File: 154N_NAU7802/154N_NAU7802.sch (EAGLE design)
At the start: 27 parts, among them IC1 MCP604SL, IC2 NAU7802SGI, J4 1725698, J5 1725698, U3 NAU7802, U4 LMV324

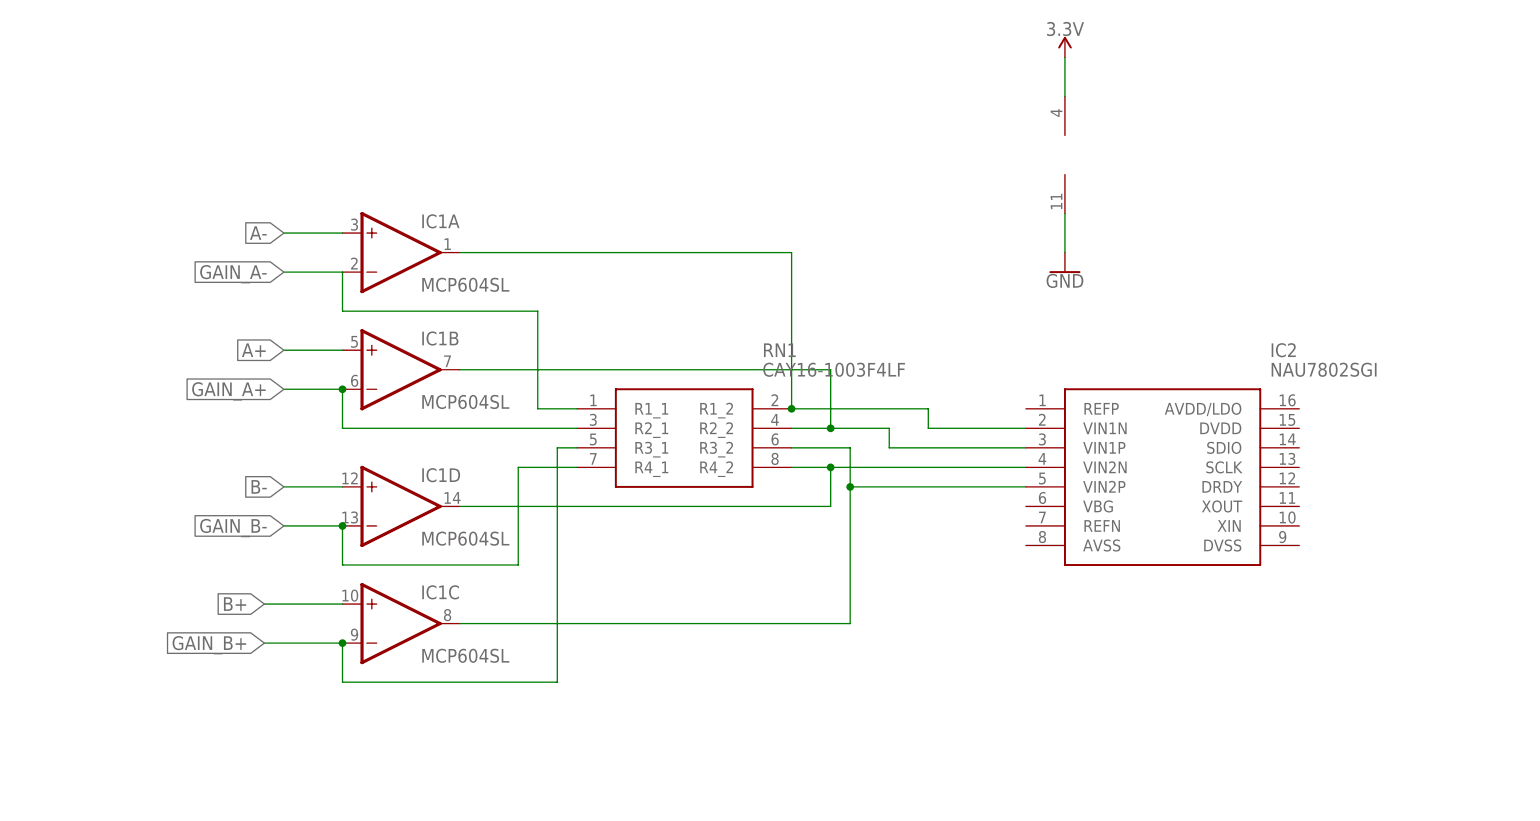
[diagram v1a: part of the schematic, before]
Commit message: Lagopus 3 mm.
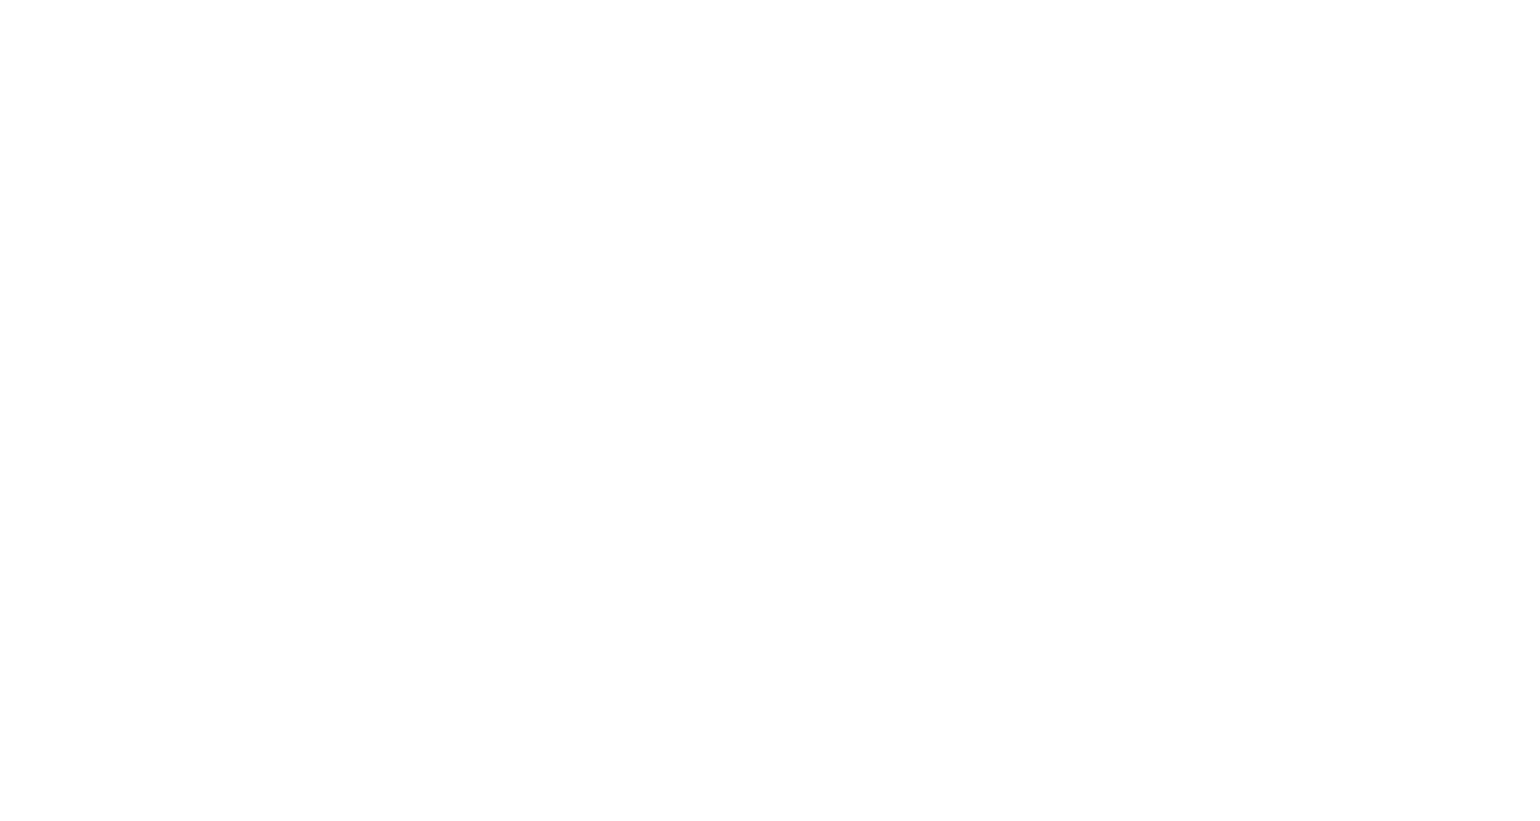
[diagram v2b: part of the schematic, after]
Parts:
- removed IC1: MCP604SL, linear:MCP604SL
- removed IC2: NAU7802SGI, NAU7802SGI:NAU7802SGI
- removed RN1: CAY16-1003F4LF, CAY16-1003F4LF:CAY16-1003F4LF
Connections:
- removed net N$16: IC1C.OUT, IC2.VIN2P, RN1.R3_2
- removed net N$5: IC1A.OUT, IC2.VIN1N, RN1.R1_2
- removed net N$7: IC1B.OUT, IC2.VIN1P, RN1.R2_2
- removed net N$8: IC1D.OUT, IC2.VIN2N, RN1.R4_2
- net 3.3V: no longer IC1P.V+
- net A+: no longer IC1B.+IN
- net A-: no longer IC1A.+IN
- net B+: no longer IC1C.+IN
- net B-: no longer IC1D.+IN
- net GAIN_A+: no longer IC1B.-IN, RN1.R2_1
- net GAIN_A-: no longer IC1A.-IN, RN1.R1_1
- net GAIN_B+: no longer IC1C.-IN, RN1.R3_1
- net GAIN_B-: no longer IC1D.-IN, RN1.R4_1
- net GND: no longer IC1P.V-
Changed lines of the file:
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@@
 <part name="SUPPLY2" library="SparkFun-PowerSymbols" library_urn="urn:adsk.eagle:library:530" deviceset="3.3V" device=""/>
 <part name="SUPPLY3" library="SparkFun-PowerSymbols" library_urn="urn:adsk.eagle:library:530" deviceset="3.3V" device=""/>
-<part name="IC1" library="linear" library_urn="urn:adsk.eagle:library:262" deviceset="MCP604" device="SL" package3d_urn="urn:adsk.eagle:package:16406/2"/>
-<part name="SUPPLY4" library="SparkFun-PowerSymbols" library_urn="urn:adsk.eagle:library:530" deviceset="3.3V" device=""/>
-<part name="GND3" library="SparkFun-PowerSymbols" library_urn="urn:adsk.eagle:library:530" deviceset="GND" device=""/>
-<part name="IC2" library="NAU7802SGI" deviceset="NAU7802SGI" device=""/>
-<part name="RN1" library="CAY16-1003F4LF" deviceset="CAY16-1003F4LF" device=""/>
 </parts>
 <sheets>
@@
 <attribute name="VALUE" x="81.28" y="96.774" size="1.778" layer="96" font="vector" align="bottom-center"/>
 </instance>
-<instance part="IC1" gate="A" x="-2.54" y="228.6" smashed="yes">
-<attribute name="NAME" x="0" y="231.775" size="1.778" layer="95"/>
-<attribute name="VALUE" x="0" y="223.52" size="1.778" layer="96"/>
-</instance>
-<instance part="IC1" gate="P" x="83.82" y="241.3" smashed="yes"/>
-<instance part="IC1" gate="B" x="-2.54" y="213.36" smashed="yes">
-<attribute name="NAME" x="0" y="216.535" size="1.778" layer="95"/>
-<attribute name="VALUE" x="0" y="208.28" size="1.778" layer="96"/>
-</instance>
-<instance part="IC1" gate="C" x="-2.54" y="180.34" smashed="yes">
-<attribute name="NAME" x="0" y="183.515" size="1.778" layer="95"/>
-<attribute name="VALUE" x="0" y="175.26" size="1.778" layer="96"/>
-</instance>
-<instance part="IC1" gate="D" x="-2.54" y="195.58" smashed="yes">
-<attribute name="NAME" x="0" y="198.755" size="1.778" layer="95"/>
-<attribute name="VALUE" x="0" y="190.5" size="1.778" layer="96"/>
-</instance>
-<instance part="SUPPLY4" gate="G$1" x="83.82" y="254" smashed="yes">
-<attribute name="VALUE" x="83.82" y="256.794" size="1.778" layer="96" font="vector" align="bottom-center"/>
-</instance>
-<instance part="GND3" gate="1" x="83.82" y="226.06" smashed="yes">
-<attribute name="VALUE" x="83.82" y="225.806" size="1.778" layer="96" font="vector" align="top-center"/>
-</instance>
-<instance part="IC2" gate="G$1" x="78.74" y="208.28" smashed="yes">
-<attribute name="NAME" x="110.49" y="215.9" size="1.778" layer="95" align="center-left"/>
-<attribute name="VALUE" x="110.49" y="213.36" size="1.778" layer="96" align="center-left"/>
-</instance>
-<instance part="RN1" gate="G$1" x="20.32" y="208.28" smashed="yes">
-<attribute name="NAME" x="44.45" y="215.9" size="1.778" layer="95" align="center-left"/>
-<attribute name="VALUE" x="44.45" y="213.36" size="1.778" layer="96" align="center-left"/>
-</instance>
 </instances>
 <busses>
@@
 <wire x1="81.28" y1="83.82" x2="81.28" y2="81.28" width="0.1524" layer="91"/>
 </segment>
-<segment>
-<pinref part="IC1" gate="P" pin="V-"/>
-<wire x1="83.82" y1="233.68" x2="83.82" y2="228.6" width="0.1524" layer="91"/>
-<pinref part="GND3" gate="1" pin="GND"/>
-</segment>
 </net>
 <net name="SCL" class="0">
@@
 <pinref part="SUPPLY3" gate="G$1" pin="3.3V"/>
 </segment>
-<segment>
-<pinref part="IC1" gate="P" pin="V+"/>
-<wire x1="83.82" y1="248.92" x2="83.82" y2="254" width="0.1524" layer="91"/>
-<pinref part="SUPPLY4" gate="G$1" pin="3.3V"/>
-</segment>
 </net>
 <net name="INT" class="0">
@@
 <pinref part="J4" gate="G$1" pin="6"/>
 </segment>
-<segment>
-<label x="-20.32" y="182.88" size="1.778" layer="95" rot="R180" xref="yes"/>
-<pinref part="IC1" gate="C" pin="+IN"/>
-<wire x1="-10.16" y1="182.88" x2="-20.32" y2="182.88" width="0.1524" layer="91"/>
-</segment>
 </net>
 <net name="B-" class="0">
@@
 <label x="-60.96" y="35.56" size="1.27" layer="95" rot="R180" xref="yes"/>
 <pinref part="J4" gate="G$1" pin="3"/>
-</segment>
-<segment>
-<wire x1="-10.16" y1="198.12" x2="-17.78" y2="198.12" width="0.1524" layer="91"/>
-<label x="-17.78" y="198.12" size="1.778" layer="95" rot="R180" xref="yes"/>
-<pinref part="IC1" gate="D" pin="+IN"/>
 </segment>
 </net>
@@
 <pinref part="J5" gate="G$1" pin="1"/>
 </segment>
-<segment>
-<wire x1="-10.16" y1="215.9" x2="-17.78" y2="215.9" width="0.1524" layer="91"/>
-<label x="-17.78" y="215.9" size="1.778" layer="95" rot="R180" xref="yes"/>
-<pinref part="IC1" gate="B" pin="+IN"/>
-</segment>
 </net>
 <net name="A-" class="0">
@@
 <label x="-60.96" y="83.82" size="1.27" layer="95" rot="R180" xref="yes"/>
 <pinref part="J5" gate="G$1" pin="4"/>
-</segment>
-<segment>
-<wire x1="-10.16" y1="231.14" x2="-17.78" y2="231.14" width="0.1524" layer="91"/>
-<label x="-17.78" y="231.14" size="1.778" layer="95" rot="R180" xref="yes"/>
-<pinref part="IC1" gate="A" pin="+IN"/>
 </segment>
 </net>
@@
 <pinref part="J5" gate="G$1" pin="5"/>
 </segment>
-<segment>
-<wire x1="-10.16" y1="210.82" x2="-17.78" y2="210.82" width="0.1524" layer="91"/>
-<label x="-17.78" y="210.82" size="1.778" layer="95" rot="R180" xref="yes"/>
-<pinref part="IC1" gate="B" pin="-IN"/>
-<pinref part="RN1" gate="G$1" pin="R2_1"/>
-<wire x1="-10.16" y1="210.82" x2="-10.16" y2="205.74" width="0.1524" layer="91"/>
-<wire x1="-10.16" y1="205.74" x2="20.32" y2="205.74" width="0.1524" layer="91"/>
-<junction x="-10.16" y="210.82"/>
-</segment>
 </net>
 <net name="GAIN_B-" class="0">
@@
 <pinref part="J4" gate="G$1" pin="1"/>
 </segment>
-<segment>
-<wire x1="-10.16" y1="193.04" x2="-17.78" y2="193.04" width="0.1524" layer="91"/>
-<label x="-17.78" y="193.04" size="1.778" layer="95" rot="R180" xref="yes"/>
-<pinref part="IC1" gate="D" pin="-IN"/>
-<wire x1="-10.16" y1="193.04" x2="-10.16" y2="187.96" width="0.1524" layer="91"/>
-<junction x="-10.16" y="193.04"/>
-<wire x1="-10.16" y1="187.96" x2="12.7" y2="187.96" width="0.1524" layer="91"/>
-<wire x1="12.7" y1="187.96" x2="12.7" y2="200.66" width="0.1524" layer="91"/>
-<pinref part="RN1" gate="G$1" pin="R4_1"/>
-<wire x1="12.7" y1="200.66" x2="20.32" y2="200.66" width="0.1524" layer="91"/>
-</segment>
 </net>
 <net name="GAIN_B+" class="0">
@@
 <label x="-60.96" y="38.1" size="1.27" layer="95" rot="R180" xref="yes"/>
 <pinref part="J4" gate="G$1" pin="2"/>
-</segment>
-<segment>
-<label x="-20.32" y="177.8" size="1.778" layer="95" rot="R180" xref="yes"/>
-<pinref part="IC1" gate="C" pin="-IN"/>
-<wire x1="-10.16" y1="177.8" x2="-10.16" y2="172.72" width="0.1524" layer="91"/>
-<wire x1="-10.16" y1="177.8" x2="-20.32" y2="177.8" width="0.1524" layer="91"/>
-<junction x="-10.16" y="177.8"/>
-<wire x1="-10.16" y1="172.72" x2="17.78" y2="172.72" width="0.1524" layer="91"/>
-<wire x1="17.78" y1="172.72" x2="17.78" y2="203.2" width="0.1524" layer="91"/>
-<pinref part="RN1" gate="G$1" pin="R3_1"/>
-<wire x1="17.78" y1="203.2" x2="20.32" y2="203.2" width="0.1524" layer="91"/>
 </segment>
 </net>
@@
 <pinref part="J5" gate="G$1" pin="6"/>
 </segment>
-<segment>
-<wire x1="-10.16" y1="226.06" x2="-17.78" y2="226.06" width="0.1524" layer="91"/>
-<label x="-17.78" y="226.06" size="1.778" layer="95" rot="R180" xref="yes"/>
-<pinref part="IC1" gate="A" pin="-IN"/>
-<wire x1="-10.16" y1="226.06" x2="-10.16" y2="220.98" width="0.1524" layer="91"/>
-<wire x1="-10.16" y1="220.98" x2="15.24" y2="220.98" width="0.1524" layer="91"/>
-<wire x1="15.24" y1="220.98" x2="15.24" y2="208.28" width="0.1524" layer="91"/>
-<pinref part="RN1" gate="G$1" pin="R1_1"/>
-<wire x1="15.24" y1="208.28" x2="20.32" y2="208.28" width="0.1524" layer="91"/>
-</segment>
-</net>
-<net name="N$5" class="0">
-<segment>
-<pinref part="RN1" gate="G$1" pin="R1_2"/>
-<wire x1="48.26" y1="208.28" x2="48.26" y2="228.6" width="0.1524" layer="91"/>
-<pinref part="IC1" gate="A" pin="OUT"/>
-<wire x1="48.26" y1="228.6" x2="5.08" y2="228.6" width="0.1524" layer="91"/>
-<wire x1="48.26" y1="208.28" x2="66.04" y2="208.28" width="0.1524" layer="91"/>
-<junction x="48.26" y="208.28"/>
-<wire x1="66.04" y1="208.28" x2="66.04" y2="205.74" width="0.1524" layer="91"/>
-<pinref part="IC2" gate="G$1" pin="VIN1N"/>
-<wire x1="66.04" y1="205.74" x2="78.74" y2="205.74" width="0.1524" layer="91"/>
-</segment>
-</net>
-<net name="N$7" class="0">
-<segment>
-<pinref part="IC1" gate="B" pin="OUT"/>
-<wire x1="5.08" y1="213.36" x2="53.34" y2="213.36" width="0.1524" layer="91"/>
-<wire x1="53.34" y1="213.36" x2="53.34" y2="205.74" width="0.1524" layer="91"/>
-<pinref part="RN1" gate="G$1" pin="R2_2"/>
-<wire x1="53.34" y1="205.74" x2="48.26" y2="205.74" width="0.1524" layer="91"/>
-<pinref part="IC2" gate="G$1" pin="VIN1P"/>
-<wire x1="78.74" y1="203.2" x2="60.96" y2="203.2" width="0.1524" layer="91"/>
-<wire x1="60.96" y1="203.2" x2="60.96" y2="205.74" width="0.1524" layer="91"/>
-<wire x1="60.96" y1="205.74" x2="53.34" y2="205.74" width="0.1524" layer="91"/>
-<junction x="53.34" y="205.74"/>
-</segment>
-</net>
-<net name="N$8" class="0">
-<segment>
-<pinref part="IC1" gate="D" pin="OUT"/>
-<wire x1="53.34" y1="195.58" x2="5.08" y2="195.58" width="0.1524" layer="91"/>
-<pinref part="IC2" gate="G$1" pin="VIN2N"/>
-<wire x1="78.74" y1="200.66" x2="53.34" y2="200.66" width="0.1524" layer="91"/>
-<pinref part="RN1" gate="G$1" pin="R4_2"/>
-<wire x1="53.34" y1="200.66" x2="48.26" y2="200.66" width="0.1524" layer="91"/>
-<wire x1="53.34" y1="195.58" x2="53.34" y2="200.66" width="0.1524" layer="91"/>
-<junction x="53.34" y="200.66"/>
-</segment>
-</net>
-<net name="N$16" class="0">
-<segment>
-<pinref part="IC1" gate="C" pin="OUT"/>
-<wire x1="55.88" y1="180.34" x2="5.08" y2="180.34" width="0.1524" layer="91"/>
-<pinref part="IC2" gate="G$1" pin="VIN2P"/>
-<wire x1="78.74" y1="198.12" x2="55.88" y2="198.12" width="0.1524" layer="91"/>
-<pinref part="RN1" gate="G$1" pin="R3_2"/>
-<wire x1="48.26" y1="203.2" x2="55.88" y2="203.2" width="0.1524" layer="91"/>
-<wire x1="55.88" y1="203.2" x2="55.88" y2="198.12" width="0.1524" layer="91"/>
-<wire x1="55.88" y1="180.34" x2="55.88" y2="198.12" width="0.1524" layer="91"/>
-<junction x="55.88" y="198.12"/>
-</segment>
-</net>
+</net>
